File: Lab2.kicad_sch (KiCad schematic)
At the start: 10 parts, among them U1 ATmega328-P, U2 TLV2472, U3 TLE2426

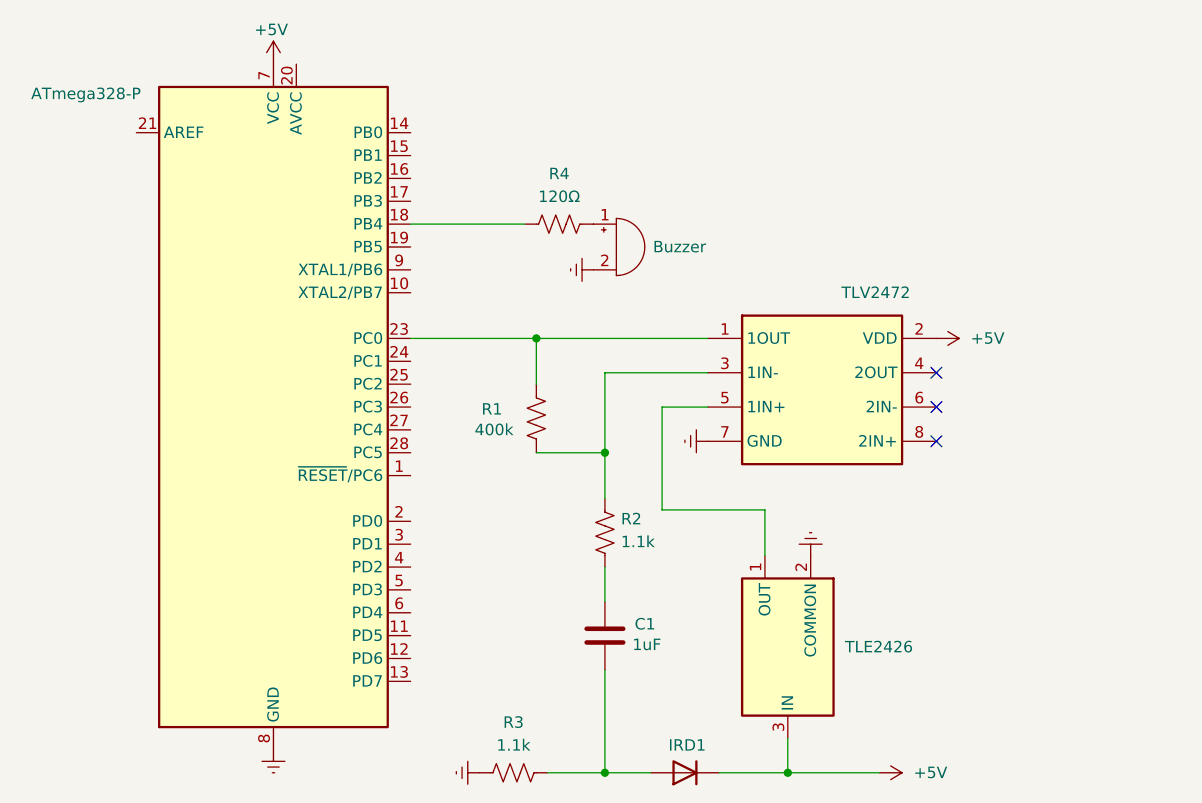
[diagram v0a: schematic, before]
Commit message: Add files via upload
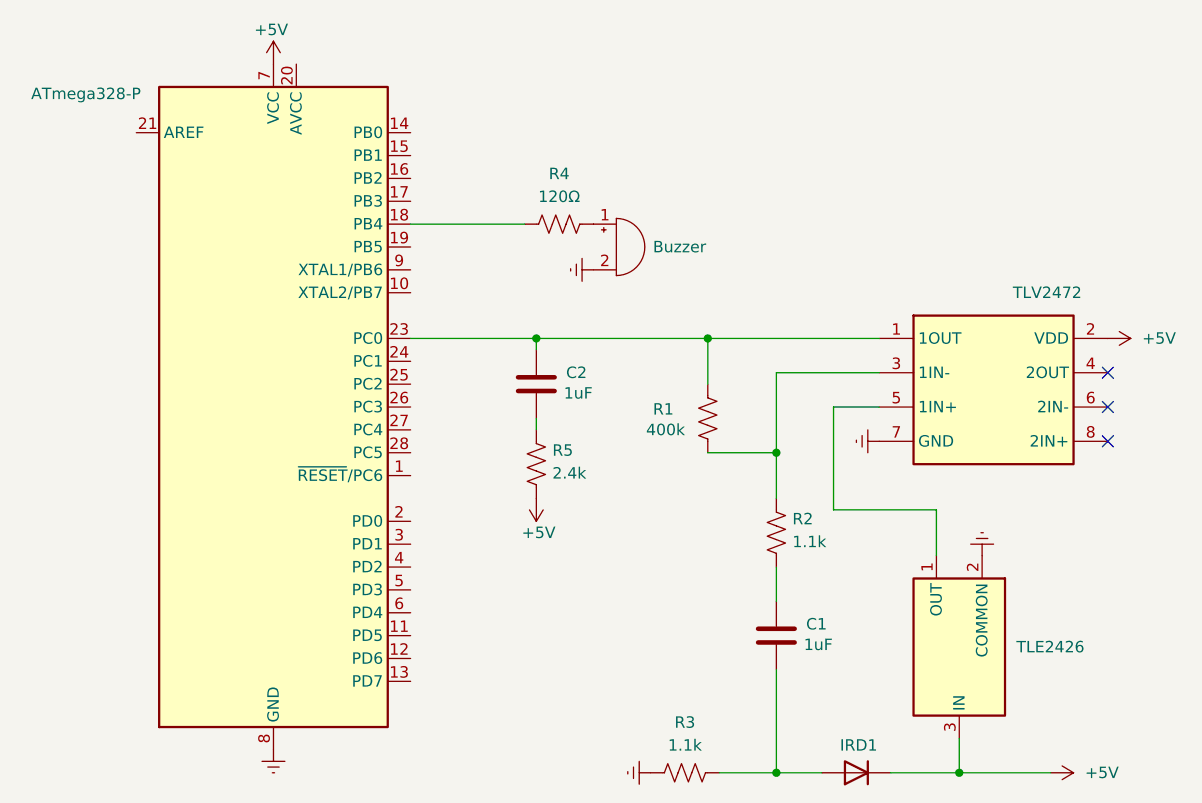
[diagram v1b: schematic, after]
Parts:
- added C2: 1uF, symbol Device:C
- added R5: 2.4k, symbol Device:R_US
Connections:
- net +5V: now also R5.2
- net at R1.1, U1.23 (PC0), U2.1 (1OUT): now also C2.1
- new net: C2.2, R5.1
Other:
- moved on the sheet: C1, IRD1, R1, R2, R3
